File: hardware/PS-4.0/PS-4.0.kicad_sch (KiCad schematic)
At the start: 71 parts, among them CN1 Conn_01x02, CN5 Conn_01x02, CN6 Conn_01x03, J1 PinSocket_02x16_P2.54mm_Verti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, K1 G2RL-2, K1 RAYEX-L90, K2 G2RL-2, K2 RAYEX-L90, Q1 IRFPE50, Q2 IRFPE50, Q3 IRFPE50, U1 TC4422/ TC4420, U4 PC817

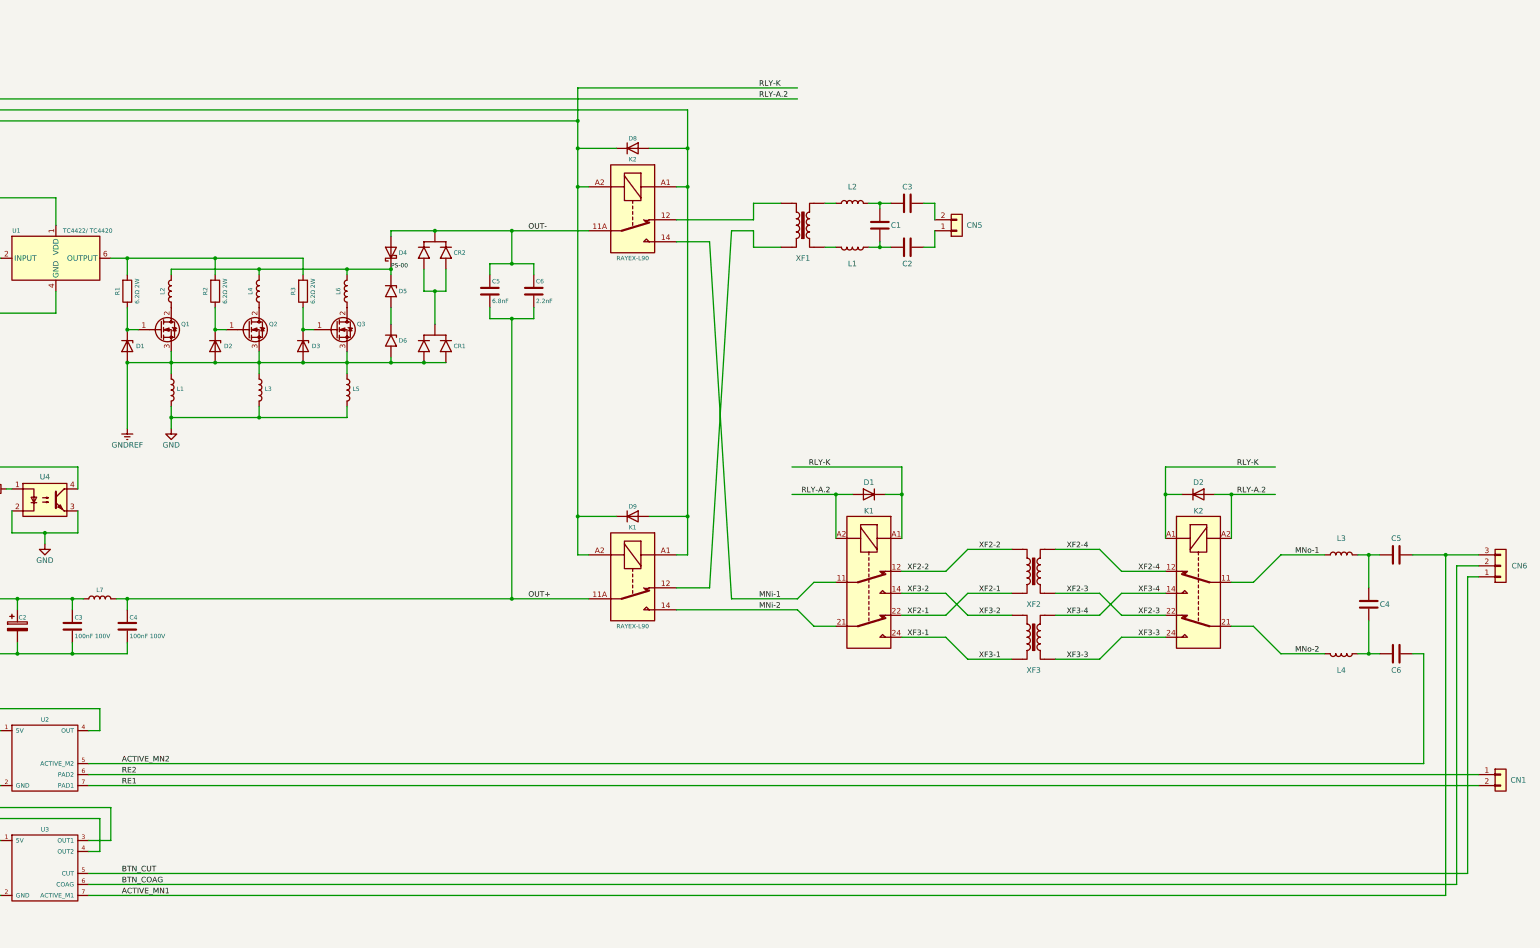
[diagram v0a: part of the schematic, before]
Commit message: modified:   .DS_Store 	new file:   CAD/enclosure.dwg 	new file:   CAD/front-panel.dwg 	new file:   CAD/socket-bipolar-v1.dwg 	new file:   CAD/socket-monopolar-v1.dwg 	new file:   CAD/socket-re-v1.dwg 	new file:   CAD/test-probe.dwg 	modified:   Ferrite Transformer Calculation.xlsx 	new file:   archive/Purchase 20260105.xlsx 	modified:   firmware/ESP32-S3 PWM/src/buzzer.cpp 	new file:   hardware/CTL-4.1/CTL-4.1-backups/CTL-4.1-2025-10-23_132246.zip 	new file:   hardware/CTL-4.1/CTL-4.1-backups/CTL-4.1-2025-11-21_160148.zip 	new file:   hardware/CTL-4.1/CTL-4.1-backups/CTL-4.1-2025-11-21_161233.zip 	new file:   hardware/CTL-4.1/CTL-4.1-backups/CTL-4.1-2025-11-21_161917.zip 	new file:   hardware/CTL-4.1/CTL-4.1-backups/CTL-4.1-2025-11-21_162924.zip 	new file:   hardware/CTL-4.1/CTL-4.1-backups/CTL-4.1-2025-11-21_163425.zip 	new file:   hardware/CTL-4.1/CTL-4.1-backups/CTL-4.1-2025-11-24_100545.zip 	new file:   hardware/CTL-4.1/CTL-4.1-backups/CTL-4.1-2026-01-01_173613.zip 	new file:   hardware/CTL-4.1/CTL-4.1-backups/CTL-4.1-2026-01-01_174207.zip 	new file:   hardware/CTL-4.1/CTL-4.1-backups/CTL-4.1-2026-01-01_174749.zip 	new file:   hardware/CTL-4.1/CTL-4.1-backups/CTL-4.1-2026-01-02_130920.zip 	new file:   hardware/CTL-4.1/CTL-4.1-backups/CTL-4.1-2026-01-06_145810.zip 	new file:   hardware/CTL-4.1/CTL-4.1-backups/CTL-4.1-2026-01-06_164111.zip 	modified:   hardware/CTL-4.1/CTL-4.1.kicad_pcb 	modified:   hardware/CTL-4.1/CTL-4.1.kicad_prl 	modified:   hardware/CTL-4.1/CTL-4.1.kicad_pro 	new file:   hardware/CTL-4.1/bom/ibom.html 	modified:   hardware/CTL-4.1/fp-info-cache 	new file:   hardware/PS-3.0/PS-3.0-backups/PS-3.0-2025-10-23_133252.zip 	new file:   hardware/PS-3.0/PS-3.0-backups/PS-3.0-2025-11-20_095956.zip 	new file:   hardware/PS-3.0/PS-3.0-backups/PS-3.0-2025-11-20_100505.zip 	deleted:    hardware/PS-4.0/PS-4.0-backups/PS-4.0-2025-10-01_154815.zip 	new file:   hardware/PS-4.0/PS-4.0-backups/PS-4.0-2025-10-23_133027.zip 	new file:   hardware/PS-4.0/PS-4.0-bac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
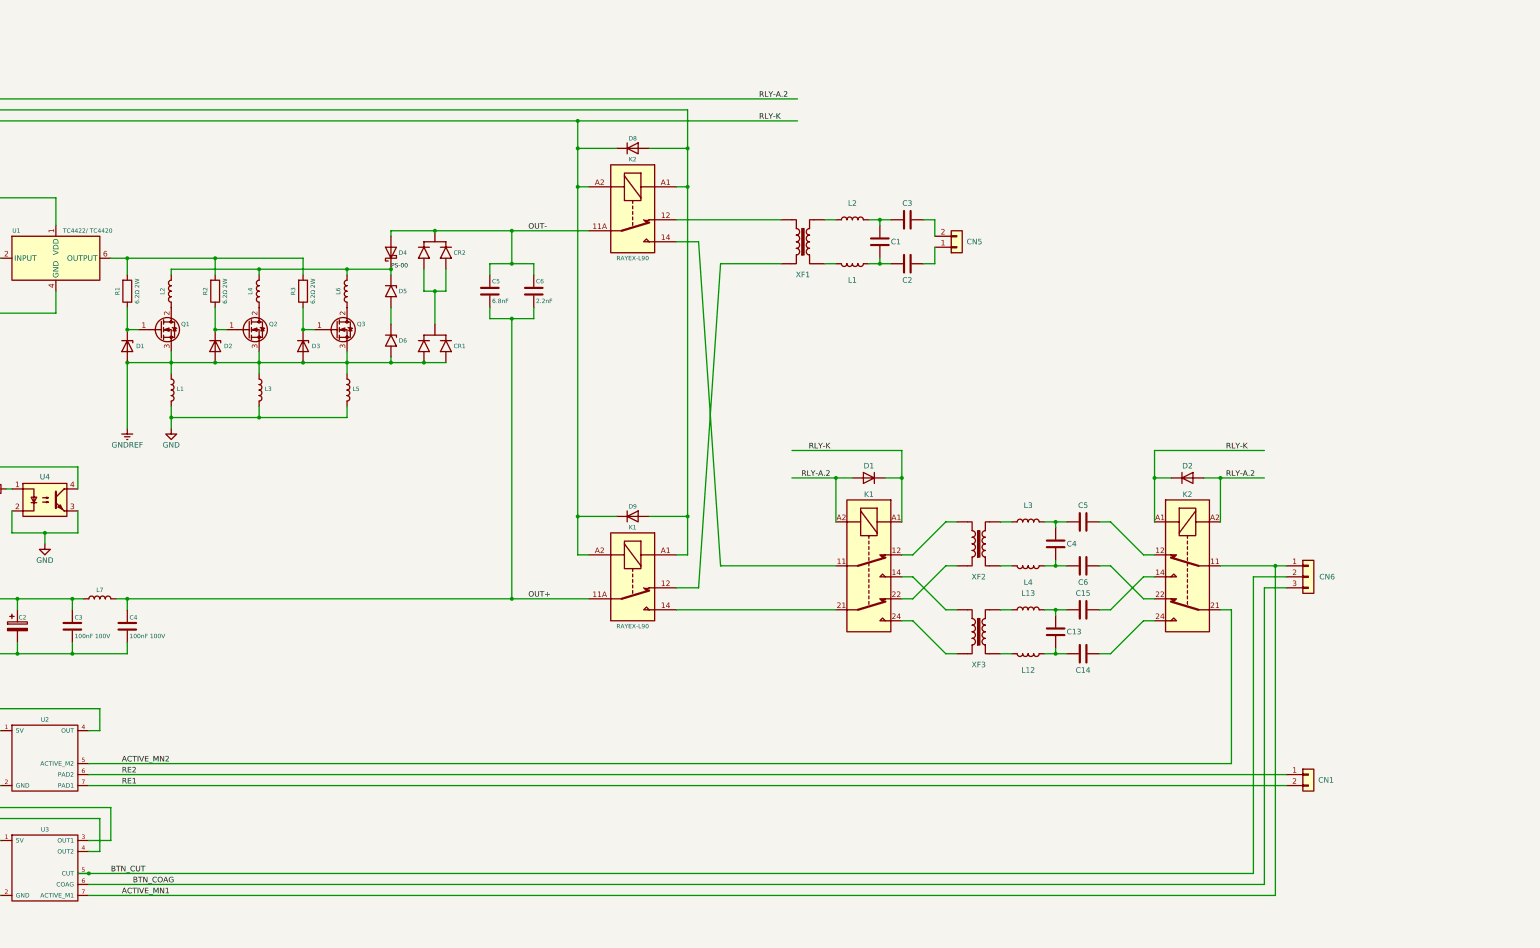
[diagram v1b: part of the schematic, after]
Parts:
- added C13: 2.7nF, Capacitor_THT:C_Rect_L18.0mm_W7.0mm_P15.00mm_FKS3_FKP3, symbol Device:C
- added C14, C15: 4.7nF, Capacitor_THT:C_Rect_L18.0mm_W7.0mm_P15.00mm_FKS3_FKP3, symbol Device:C
- added L12, L13: 29µH, Inductor_THT:L_Radial_Multilayer_D8.0mm_P12.70mm, symbol Device:L
- C1, C4: footprint Capacitor_THT:C_Axial_L12.0mm_D6.5mm_P15.00mm_Horizontal -> Capacitor_THT:C_Rect_L18.0mm_W7.0mm_P15.00mm_FKS3_FKP3
- C2, C3, C5, C6: footprint Capacitor_THT:C_Rect_L13.0mm_W8.0mm_P10.00mm_FKS3_FKP3_MKS4 -> Capacitor_THT:C_Rect_L18.0mm_W7.0mm_P15.00mm_FKS3_FKP3
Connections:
- net ACTIVE_MN1: now also CN6.1 (Pin_1), K2.11; no longer C5.2, CN6.3 (Pin_3)
- net ACTIVE_MN2: now also K2.21; no longer C6.2
- net BTN_COAG: now also CN6.3 (Pin_3); no longer CN6.2 (Pin_2)
- net BTN_CUT: now also CN6.2 (Pin_2); no longer CN6.1 (Pin_1)
- net MNi-1: no longer names the net of K1.11, K2.14
- net MNi-2: no longer names the net of K1.14, K1.21
- net MNo-1: no longer names the net of L3.1
- net MNo-1: now also XF2.3; no longer K2.11
- net MNo-2: no longer names the net of L4.1
- net MNo-2: now also XF2.4; no longer K2.21
- net XF2-1: no longer names the net of K1.22, XF2.1
- net XF2-2: no longer names the net of K1.12, XF2.2
- net XF2-3: no longer names the net of K2.22
- net XF2-3: now also C6.2; no longer XF2.4
- net XF2-4: no longer names the net of K2.12
- net XF2-4: now also C5.2; no longer XF2.3
- net XF3-1: no longer names the net of K1.24, XF3.1
- net XF3-2: no longer names the net of K1.14, XF3.2
- net XF3-3: no longer names the net of XF3.4
- net XF3-3: now also L12.1; no longer K2.24
- net XF3-4: no longer names the net of K2.14
- net XF3-4: now also C15.2; no longer XF3.3
- new net: C13.2, C14.1, L12.2
- new net: C13.1, C15.1, L13.2
- new net: C14.2, K2.24
- new net: L13.1, XF3.3
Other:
- moved on the sheet: C1, C2, C3, C4, C5, C6, CN1, CN5, CN6, D1, D2, K1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
